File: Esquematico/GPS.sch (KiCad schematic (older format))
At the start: 1 part

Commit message: Add files via upload
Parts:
- removed IC?: NEO-6M-0-001, NEO6M0001, symbol NEO-6M-0-001:NEO-6M-0-001
- added J?: Conn_GPS, symbol Connector:Conn_01x04_Female
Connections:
- net labels added: 3V3, RXD1GPS, TXD1GPS
- net labels removed: +3.3V, Rx, Tx
- wire segments 7 -> 4
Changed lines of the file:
@@
 $Descr A4 11693 8268
 encoding utf-8
-Sheet 1 1
+Sheet 8 8
 Title ""
 Date ""
@@
 Comment4 ""
 $EndDescr
-Text GLabel 2750 3350 0    50   Input ~ 0
-Tx
-Text GLabel 2750 3500 0    50   Input ~ 0
-Rx
-Wire Wire Line
-	2850 3400 2850 3350
-Wire Wire Line
-	2850 3350 2750 3350
-Wire Wire Line
-	3350 3500 2750 3500
-Wire Wire Line
-	3350 3400 2850 3400
 $Comp
-L NEO-6M-0-001:NEO-6M-0-001 IC?
-U 1 1 6193A28E
-P 3350 2700
-F 0 "IC?" H 4300 2965 50  0000 C CNN
-F 1 "NEO-6M-0-001" H 4300 2874 50  0000 C CNN
-F 2 "NEO6M0001" H 5100 2800 50  0001 L CNN
-F 3 "https://www.u-blox.com/sites/default/files/products/documents/NEO-6_DataSheet_%28GPS.G6-HW-09005%29.pdf" H 5100 2700 50  0001 L CNN
-F 4 "GPS Module" H 5100 2600 50  0001 L CNN "Description"
-F 5 "2.6" H 5100 2500 50  0001 L CNN "Height"
-F 6 "U-Blox" H 5100 2400 50  0001 L CNN "Manufacturer_Name"
-F 7 "NEO-6M-0-001" H 5100 2300 50  0001 L CNN "Manufacturer_Part_Number"
-F 8 "" H 5100 2200 50  0001 L CNN "Mouser Part Number"
-F 9 "" H 5100 2100 50  0001 L CNN "Mouser Price/Stock"
-F 10 "" H 5100 2000 50  0001 L CNN "Arrow Part Number"
-F 11 "" H 5100 1900 50  0001 L CNN "Arrow Price/Stock"
-	1    3350 2700
+L Connector:Conn_01x04_Female J?
+U 1 1 61B217C9
+P 6150 3050
+F 0 "J?" H 6178 3026 50  0000 L CNN
+F 1 "Conn_GPS" H 6178 2935 50  0000 L CNN
+F 2 "" H 6150 3050 50  0001 C CNN
+F 3 "~" H 6150 3050 50  0001 C CNN
+	1    6150 3050
 	1    0    0    -1
 $EndComp
+Text HLabel 5800 2950 0    50   Input ~ 0
+3V3
+Text HLabel 5800 3050 0    50   Input ~ 0
+RXD1GPS
+Text HLabel 5800 3150 0    50   Input ~ 0
+TXD1GPS
 $Comp
-L power:+3.3V #PWR?
-U 1 1 61B02823
-P 2450 3700
-F 0 "#PWR?" H 2450 3550 50  0001 C CNN
-F 1 "+3.3V" H 2465 3873 50  0000 C CNN
-F 2 "" H 2450 3700 50  0001 C CNN
-F 3 "" H 2450 3700 50  0001 C CNN
-	1    2450 3700
+L power:GND #PWR?
+U 1 1 61B226F5
+P 5800 3250
+F 0 "#PWR?" H 5800 3000 50  0001 C CNN
+F 1 "GND" H 5805 3077 50  0000 C CNN
+F 2 "" H 5800 3250 50  0001 C CNN
+F 3 "" H 5800 3250 50  0001 C CNN
+	1    5800 3250
 	1    0    0    -1
 $EndComp
 Wire Wire Line
-	2450 3700 3350 3700
-$Comp
-L power:GND #PWR?
-U 1 1 61B0654F
-P 3350 4000
-F 0 "#PWR?" H 3350 3750 50  0001 C CNN
-F 1 "GND" H 3355 3827 50  0000 C CNN
-F 2 "" H 3350 4000 50  0001 C CNN
-F 3 "" H 3350 4000 50  0001 C CNN
-	1    3350 4000
-	1    0    0    -1
-$EndComp
+	5800 2950 5950 2950
 Wire Wire Line
-	3350 4050 3350 4000
-Connection ~ 3350 4000
+	5800 3050 5950 3050
 Wire Wire Line
-	3350 4000 3350 3800
+	5800 3150 5950 3150
+Wire Wire Line
+	5800 3250 5950 3250
 $EndSCHEMATC

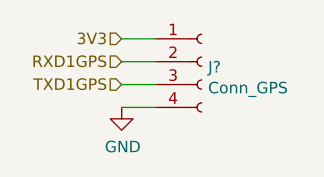
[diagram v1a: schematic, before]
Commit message: Foot prints
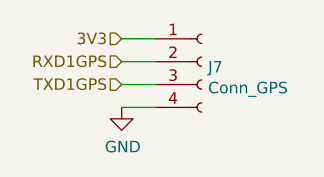
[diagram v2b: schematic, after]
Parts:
- gave numbers to parts that had none: 1
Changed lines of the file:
@@
 $EndDescr
 $Comp
-L Connector:Conn_01x04_Female J?
+L Connector:Conn_01x04_Female J7
 U 1 1 61B217C9
 P 6150 3050
-F 0 "J?" H 6178 3026 50  0000 L CNN
+F 0 "J7" H 6178 3026 50  0000 L CNN
 F 1 "Conn_GPS" H 6178 2935 50  0000 L CNN
 F 2 "" H 6150 3050 50  0001 C CNN
@@
 TXD1GPS
 $Comp
-L power:GND #PWR?
+L power:GND #PWR0119
 U 1 1 61B226F5
 P 5800 3250
-F 0 "#PWR?" H 5800 3000 50  0001 C CNN
+F 0 "#PWR0119" H 5800 3000 50  0001 C CNN
 F 1 "GND" H 5805 3077 50  0000 C CNN
 F 2 "" H 5800 3250 50  0001 C CNN

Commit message: Carga elementos PCB
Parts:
- J7: footprint (none) -> Connector_PinSocket_2.54mm:PinSocket_1x04_P2.54mm_Vertical
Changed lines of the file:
@@
 $Descr A4 11693 8268
 encoding utf-8
-Sheet 8 8
+Sheet 7 8
 Title ""
 Date ""
@@
 F 0 "J7" H 6178 3026 50  0000 L CNN
 F 1 "Conn_GPS" H 6178 2935 50  0000 L CNN
-F 2 "" H 6150 3050 50  0001 C CNN
+F 2 "Connector_PinSocket_2.54mm:PinSocket_1x04_P2.54mm_Vertical" H 6150 3050 50  0001 C CNN
 F 3 "~" H 6150 3050 50  0001 C CNN
 	1    6150 3050
